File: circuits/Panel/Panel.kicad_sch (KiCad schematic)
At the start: 14 parts

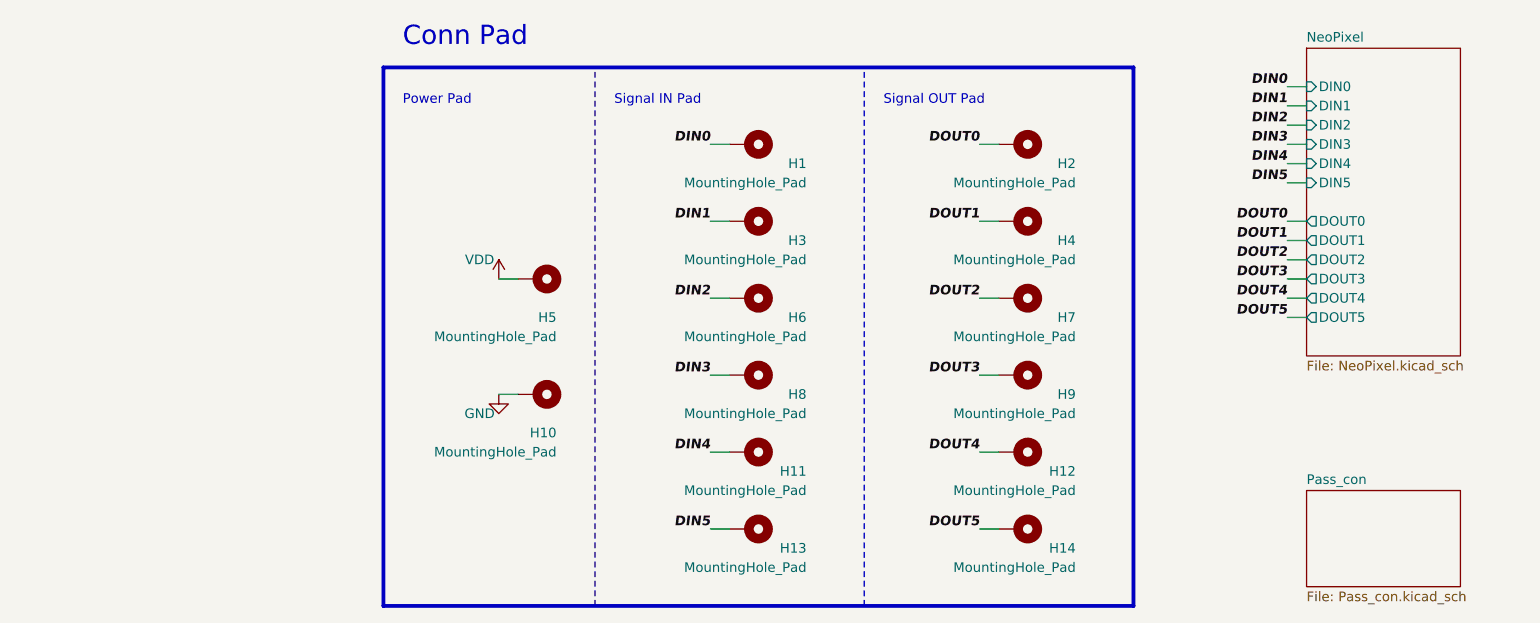
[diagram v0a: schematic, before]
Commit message: 配線おけ
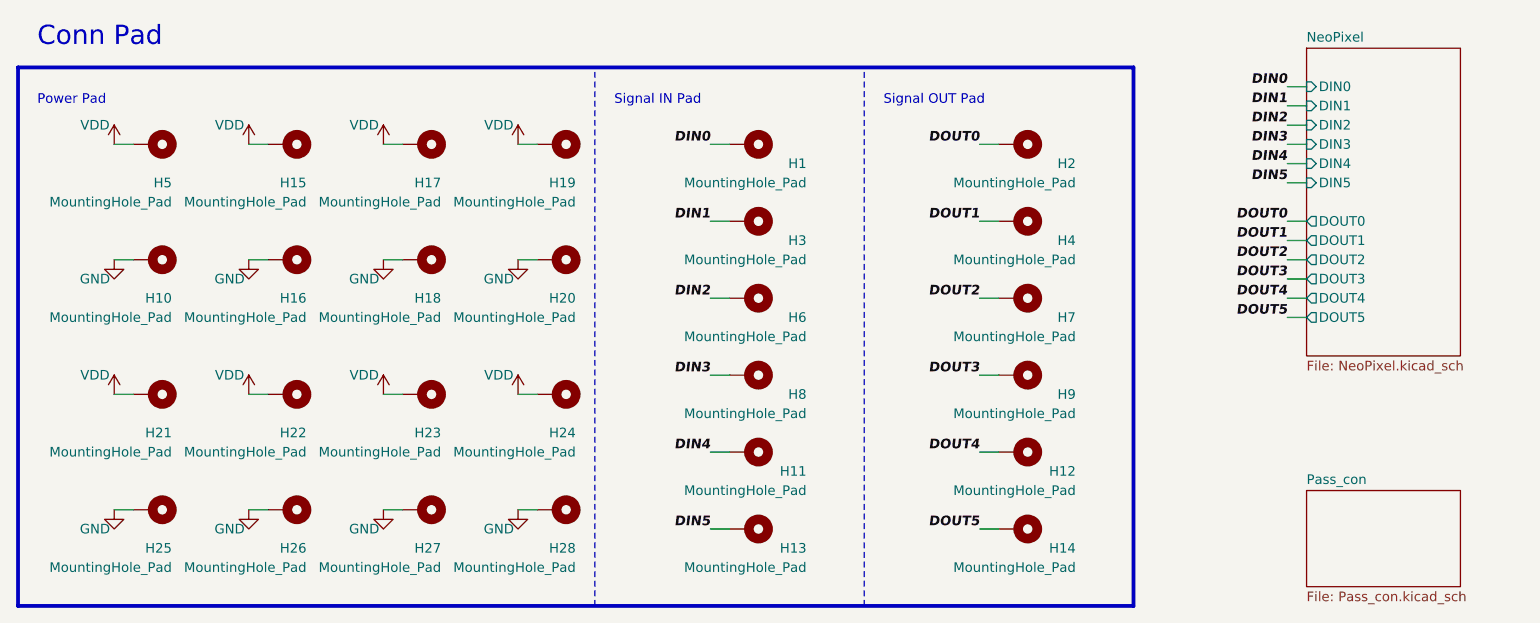
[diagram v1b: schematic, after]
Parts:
- added H15, H16, H17, H18, H19, H20, H21, H22, H23, H24, H25, H26, H27, H28: MountingHole_Pad, TestPoint:TestPoint_Pad_4.0x4.0mm, symbol Mechanical:MountingHole_Pad
- H10, H5: footprint TestPoint:TestPoint_Pad_D3.0mm -> TestPoint:TestPoint_Pad_4.0x4.0mm
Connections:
- net GND: now also H16.1, H18.1, H20.1, H25.1, H26.1, H27.1, H28.1
- net VDD: now also H15.1, H17.1, H19.1, H21.1, H22.1, H23.1, H24.1
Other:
- moved on the sheet: H10, H5
